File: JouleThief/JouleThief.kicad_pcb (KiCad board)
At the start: 2 copper layers, 8 parts, among them J1 Screw_Terminal_01x02, J2 Screw_Terminal_01x02, Q1 BC547, Q2 BC547

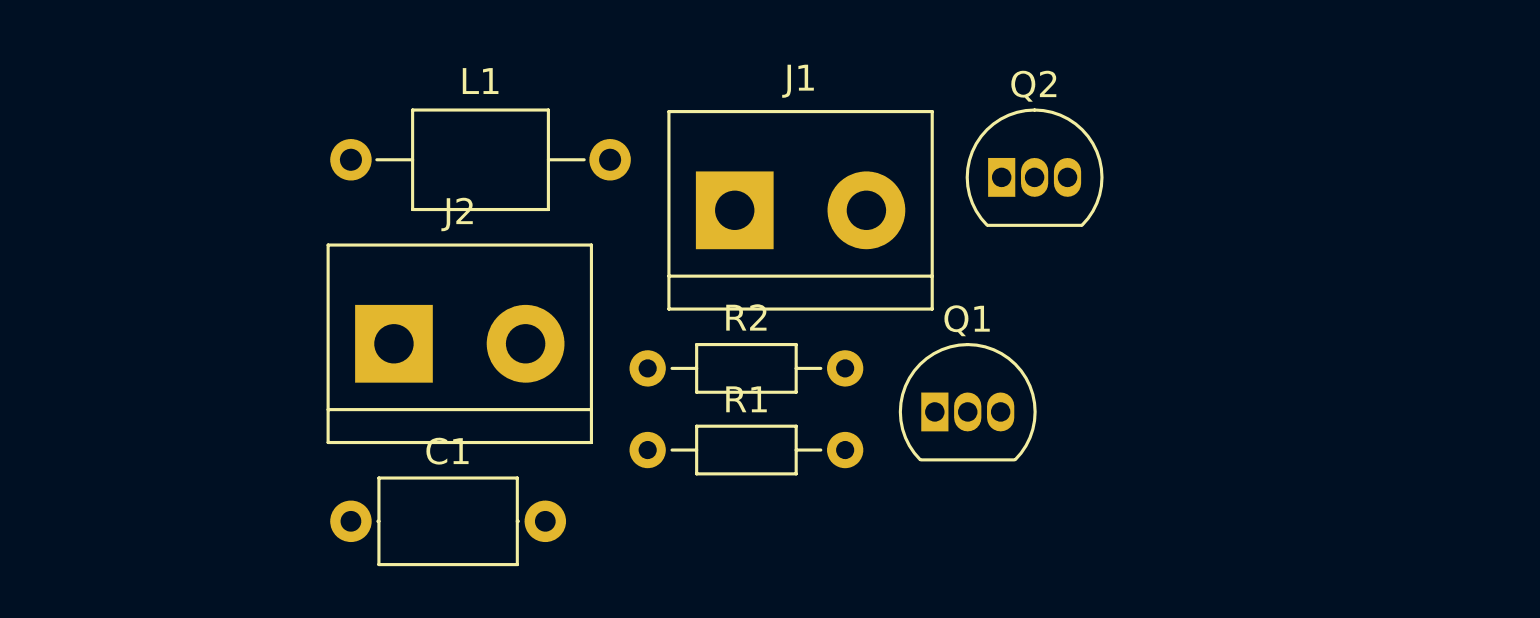
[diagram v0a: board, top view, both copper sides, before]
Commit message: Finished PCB
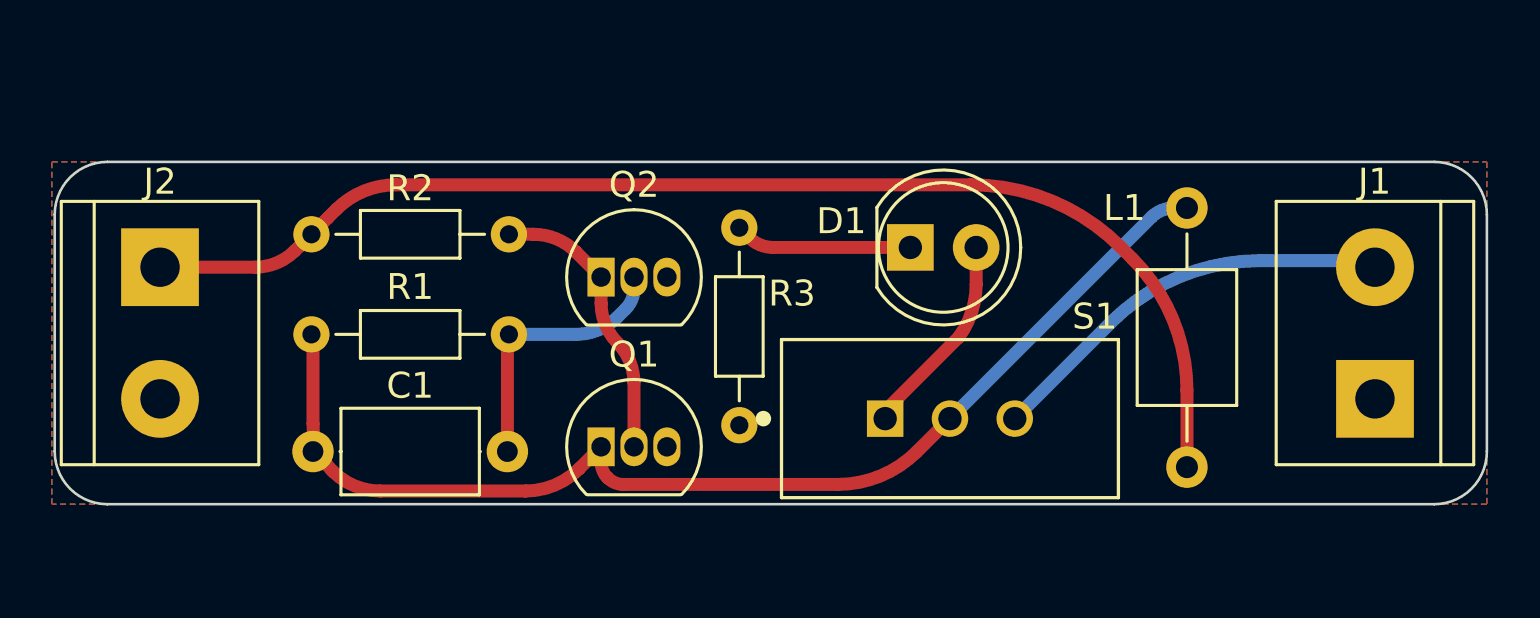
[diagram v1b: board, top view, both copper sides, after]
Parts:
- added D1: LED, LED_THT:LED_D5.0mm_Clear, F.Cu at (151.4, 95.2)
- added R3: 300, Resistor_THT:R_Axial_DIN0204_L3.6mm_D1.6mm_P7.62mm_Horizontal, F.Cu at (144.8, 94.5)
- added S1: SWITCH-SPDT-PTH-11.6X4.0MM-KIT, SnapEDA Library:SW_1825159-1, F.Cu at (152.9, 101.9)
- moved L1 32.3 mm to (162.1, 93.7), turned to -90 degrees
- moved J1 25.8 mm to (169.3, 101.1), turned to 90 degrees
- moved Q2 15.9 mm to (139.4, 96.4)
- moved R2 14.0 mm to (128.3, 94.7)
- moved R1 13.7 mm to (128.3, 98.6)
- moved Q1 12.9 mm to (139.4, 102.9)
- moved J2 9.50 mm to (122.4, 96.0), turned to -90 degrees
- moved C1 3.06 mm to (128.3, 103.1)
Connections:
- J1 pad 2: Net-(C1-Pad1) -> Net-(J1-Pad2)
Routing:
- net Net-(J2-Pad1): track 0.00 -> 47.9 mm
- net Net-(C1-Pad1): track 0.00 -> 45.0 mm
- net Net-(J1-Pad2): track 0.00 -> 16.3 mm
- net Net-(Q1-Pad2): track 0.00 -> 11.0 mm
- net Net-(C1-Pad2): track 0.00 -> 10.7 mm
- net Net-(D1-Pad2): track 0.00 -> 7.90 mm
- net Net-(D1-Pad1): track 0.00 -> 6.85 mm
- added copper zone on B.Cu, net GND
- added copper zone on F.Cu, net GND
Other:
- board outline added: 55.3 x 13.2 mm
